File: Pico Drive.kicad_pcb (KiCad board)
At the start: 2 copper layers, 100.3 x 102.2 mm, 23 parts, among them J1 Conn_01x06_Male, J2 Conn_01x08, J3 Conn_01x02_Male, J4 Conn_01x02_Male, SW1 Reset, U1 Pico, U2 74AXP1T45GWH, U3 74AHCT1G125, U4 OLED-I2C-Module-Aliexpress

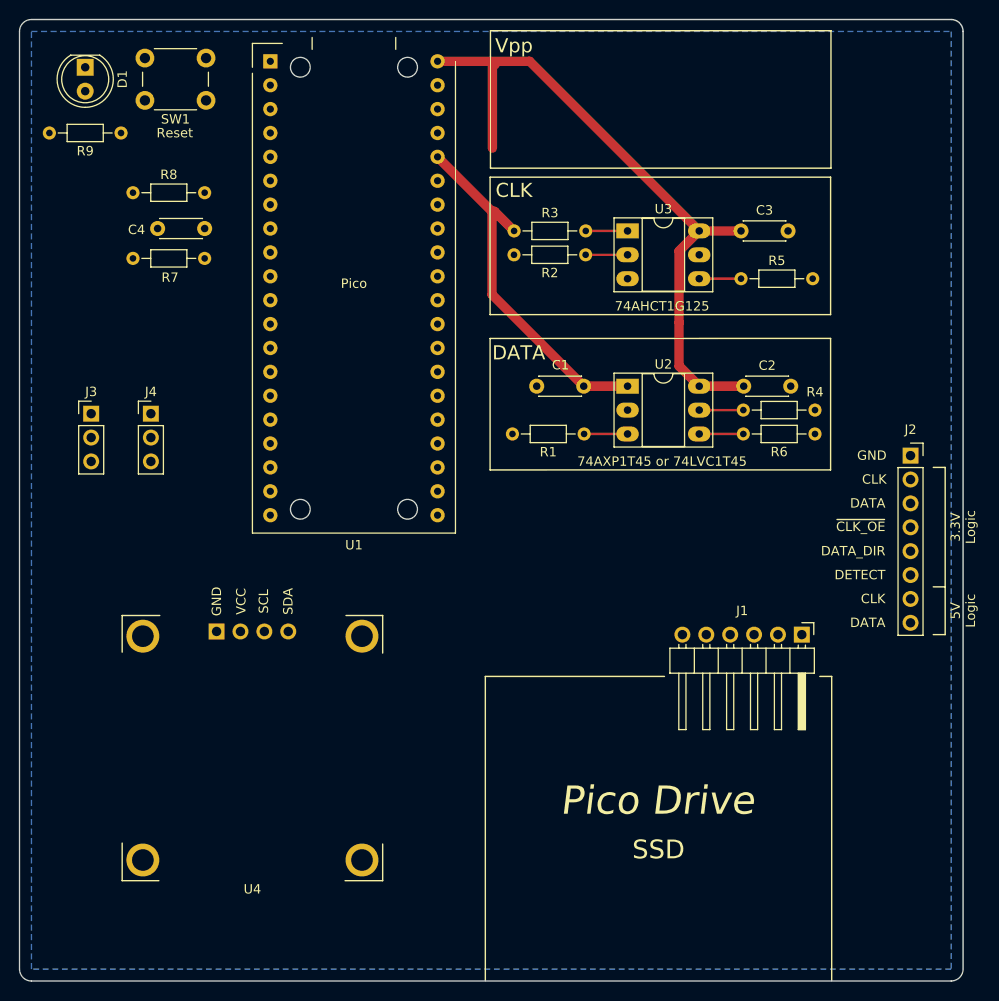
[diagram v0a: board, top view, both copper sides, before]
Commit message: Shifted bits around, ran power, added cutout
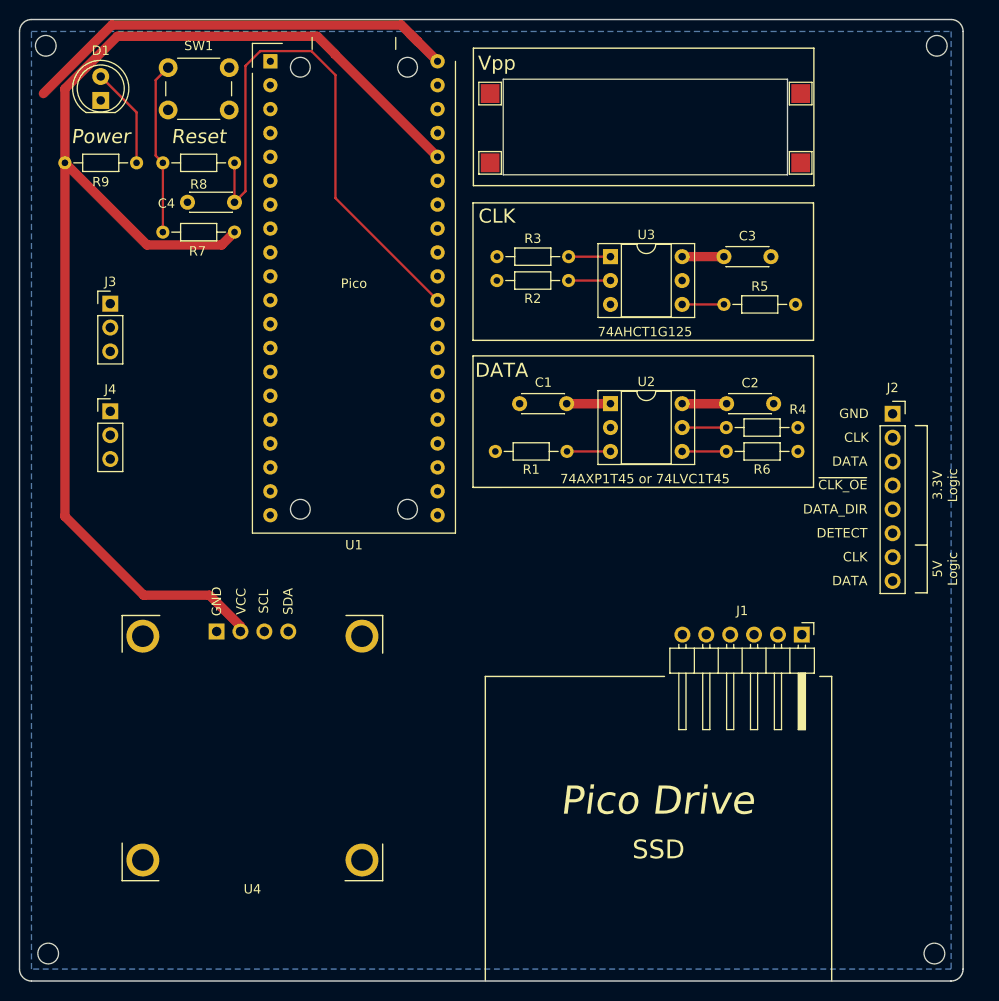
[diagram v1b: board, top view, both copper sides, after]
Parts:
- added H1: MountingHole, MountingHole:MountingHole_2.2mm_M2, F.Cu at (115.3, 18.0)
- added H2: MountingHole, MountingHole:MountingHole_2.2mm_M2, F.Cu at (20.6, 18.0)
- added H3: MountingHole, MountingHole:MountingHole_2.2mm_M2, F.Cu at (20.8, 114.6)
- added H4: MountingHole, MountingHole:MountingHole_2.2mm_M2, F.Cu at (115.1, 114.6)
- added REF**: TestPoint_Pad_2.0x2.0mm, TestPoint:TestPoint_Pad_2.0x2.0mm, F.Cu at (100.8, 30.5)
- added REF**: TestPoint_Pad_2.0x2.0mm, TestPoint:TestPoint_Pad_2.0x2.0mm, F.Cu at (100.8, 23.1)
- added REF**: TestPoint_Pad_2.0x2.0mm, TestPoint:TestPoint_Pad_2.0x2.0mm, F.Cu at (67.8, 23.1)
- added REF**: TestPoint_Pad_2.0x2.0mm, TestPoint:TestPoint_Pad_2.0x2.0mm, F.Cu at (67.8, 30.5)
- SW1: footprint Button_Switch_THT:SW_PUSH_6mm -> Button_Switch_THT:SW_PUSH_6mm_H4.3mm
- U2, U3: footprint Package_DIP:DIP-6_W7.62mm_Socket_LongPads -> Package_DIP:DIP-6_W7.62mm_Socket
- moved J3 11.9 mm to (27.4, 45.5)
- moved R7 11.2 mm to (40.6, 37.8), turned to 180 degrees
- moved R9 6.76 mm to (22.6, 30.5), turned to 0 degrees
- moved J2 4.84 mm to (110.6, 57.2)
- moved R8 4.49 mm to (33.0, 30.5)
- moved J4 4.33 mm to (27.4, 56.9)
- moved C4 4.23 mm to (40.6, 34.7)
- moved D1 3.89 mm to (26.4, 23.8), turned to 90 degrees
- moved C3 3.28 mm to (92.7, 40.5)
- moved R5 3.28 mm to (92.7, 45.5)
- moved U3 3.28 mm to (80.6, 40.5)
- moved R2 3.28 mm to (76.2, 43.0)
- moved R3 3.28 mm to (68.6, 40.5)
- moved SW1 2.67 mm to (40.1, 24.9)
- moved R1 2.60 mm to (76.0, 61.2)
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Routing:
- net +3V3: track 38.7 -> 143.7 mm
- net /~{RUN}: track 0.00 -> 58.9 mm
- net Net-(R7-Pad2): track 0.00 -> 18.4 mm
- net +5V: track 71.9 -> 57.0 mm
- net Net-(D1-Pad2): track 0.00 -> 10.8 mm
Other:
- outline, holes or cut-outs redrawn
- board text added: "Power"
